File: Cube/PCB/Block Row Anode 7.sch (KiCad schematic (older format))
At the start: 10 parts, among them U6 SN74HC595

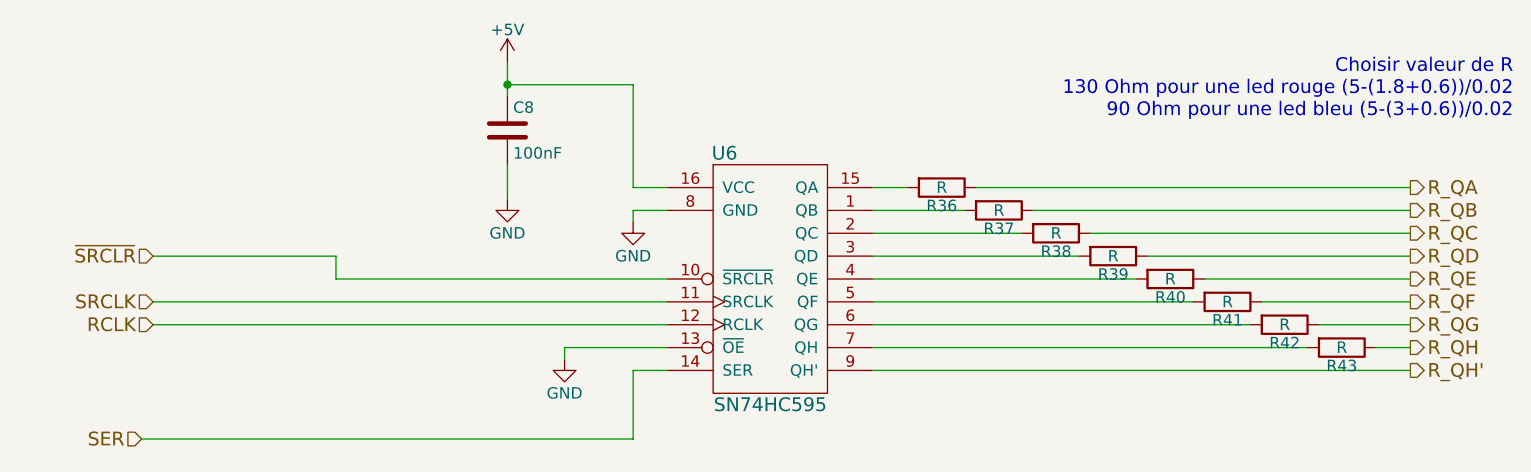
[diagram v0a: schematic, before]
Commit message: Update
Update
Add New restistor in Base Q1, Q2, Q3, Q4, Q5, Q6, Q7, Q8
New version PCB
New rename components
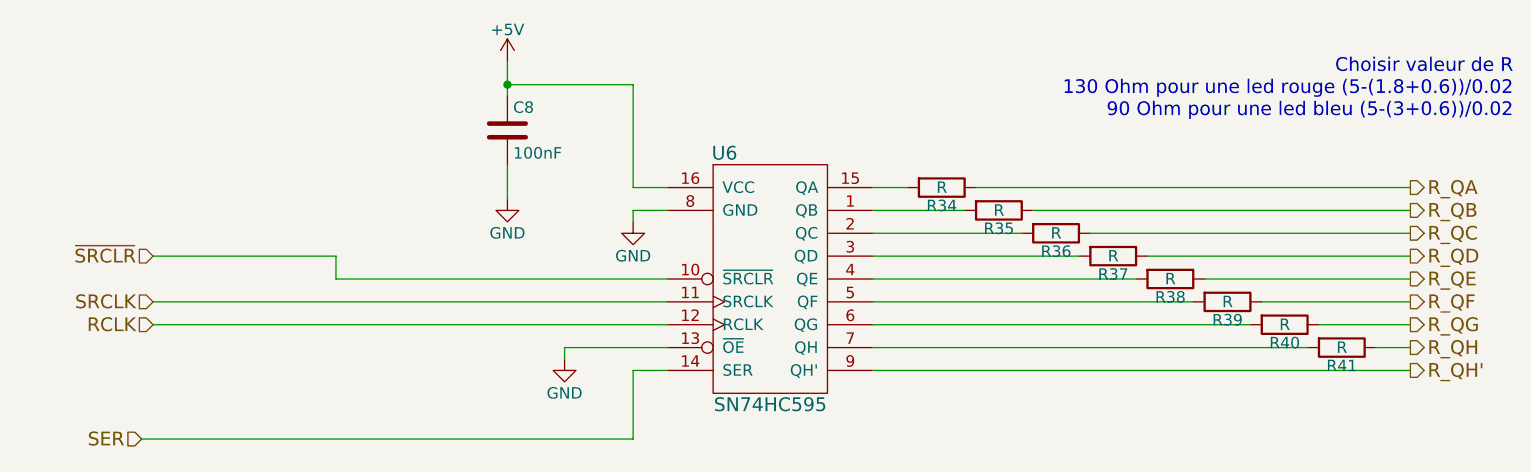
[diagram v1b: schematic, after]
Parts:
- renumbered R36 to R34, R37 to R35, R38 to R36, R39 to R37, R40 to R38, R41 to R39, R42 to R40, R43 to R41
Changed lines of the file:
@@
 R_QH'
 $Comp
-L R R36
+L R R34
 U 1 1 5B23668E
 P 5650 3250
-F 0 "R36" V 5730 3250 50  0000 C CNN
+F 0 "R34" V 5730 3250 50  0000 C CNN
 F 1 "R" V 5650 3250 50  0000 C CNN
 F 2 "alex-library:R_Axial_Long6.3mm_Dia2.5mm_Pas15.24mm_Horizontal" V 5580 3250 50  0001 C CNN
@@
 $EndComp
 $Comp
-L R R37
+L R R35
 U 1 1 5B23668F
 P 5900 3350
-F 0 "R37" V 5980 3350 50  0000 C CNN
+F 0 "R35" V 5980 3350 50  0000 C CNN
 F 1 "R" V 5900 3350 50  0000 C CNN
 F 2 "alex-library:R_Axial_Long6.3mm_Dia2.5mm_Pas15.24mm_Horizontal" V 5830 3350 50  0001 C CNN
@@
 $EndComp
 $Comp
-L R R38
+L R R36
 U 1 1 5B236690
 P 6150 3450
-F 0 "R38" V 6230 3450 50  0000 C CNN
+F 0 "R36" V 6230 3450 50  0000 C CNN
 F 1 "R" V 6150 3450 50  0000 C CNN
 F 2 "alex-library:R_Axial_Long6.3mm_Dia2.5mm_Pas15.24mm_Horizontal" V 6080 3450 50  0001 C CNN
@@
 $EndComp
 $Comp
-L R R39
+L R R37
 U 1 1 5B236691
 P 6400 3550
-F 0 "R39" V 6480 3550 50  0000 C CNN
+F 0 "R37" V 6480 3550 50  0000 C CNN
 F 1 "R" V 6400 3550 50  0000 C CNN
 F 2 "alex-library:R_Axial_Long6.3mm_Dia2.5mm_Pas15.24mm_Horizontal" V 6330 3550 50  0001 C CNN
@@
 $EndComp
 $Comp
-L R R40
+L R R38
 U 1 1 5B236692
 P 6650 3650
-F 0 "R40" V 6730 3650 50  0000 C CNN
+F 0 "R38" V 6730 3650 50  0000 C CNN
 F 1 "R" V 6650 3650 50  0000 C CNN
 F 2 "alex-library:R_Axial_Long6.3mm_Dia2.5mm_Pas15.24mm_Horizontal" V 6580 3650 50  0001 C CNN
@@
 $EndComp
 $Comp
-L R R41
+L R R39
 U 1 1 5B236693
 P 6900 3750
-F 0 "R41" V 6980 3750 50  0000 C CNN
+F 0 "R39" V 6980 3750 50  0000 C CNN
 F 1 "R" V 6900 3750 50  0000 C CNN
 F 2 "alex-library:R_Axial_Long6.3mm_Dia2.5mm_Pas15.24mm_Horizontal" V 6830 3750 50  0001 C CNN
@@
 $EndComp
 $Comp
-L R R42
+L R R40
 U 1 1 5B236694
 P 7150 3850
-F 0 "R42" V 7230 3850 50  0000 C CNN
+F 0 "R40" V 7230 3850 50  0000 C CNN
 F 1 "R" V 7150 3850 50  0000 C CNN
 F 2 "alex-library:R_Axial_Long6.3mm_Dia2.5mm_Pas15.24mm_Horizontal" V 7080 3850 50  0001 C CNN
@@
 	5350 3850 7000 3850
 $Comp
-L R R43
+L R R41
 U 1 1 5B236695
 P 7400 3950
-F 0 "R43" V 7480 3950 50  0000 C CNN
+F 0 "R41" V 7480 3950 50  0000 C CNN
 F 1 "R" V 7400 3950 50  0000 C CNN
 F 2 "alex-library:R_Axial_Long6.3mm_Dia2.5mm_Pas15.24mm_Horizontal" V 7330 3950 50  0001 C CNN
